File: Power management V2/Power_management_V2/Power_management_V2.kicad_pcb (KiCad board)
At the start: 4 copper layers, 76.5 x 66 mm, 60 parts, among them J2 1722861104, U1 SIC437AED, U2 SIC437AED, U3 TPS3711DDCR

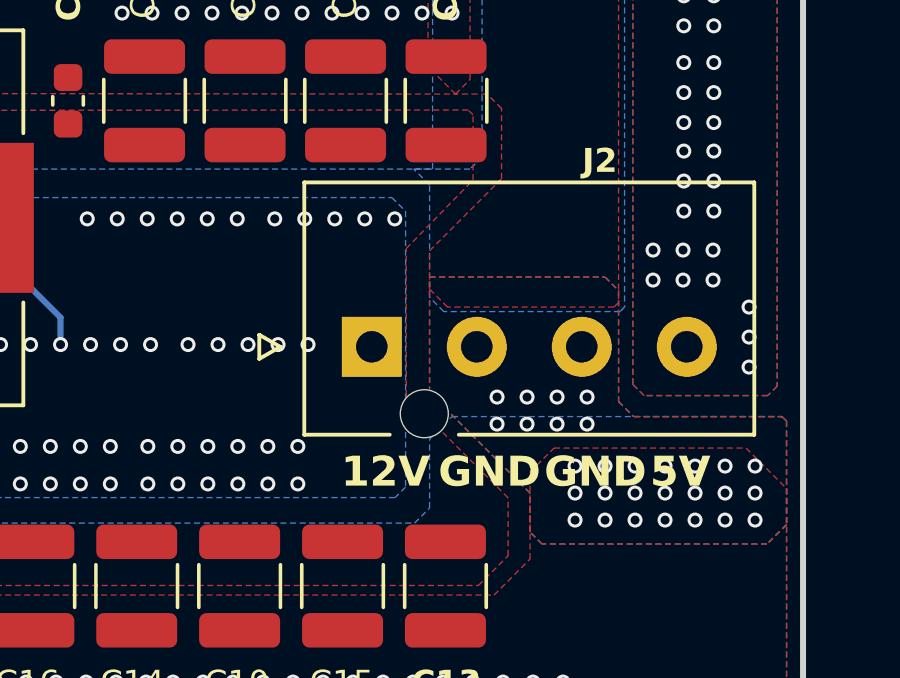
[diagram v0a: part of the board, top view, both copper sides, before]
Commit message: cap nhat 26/2
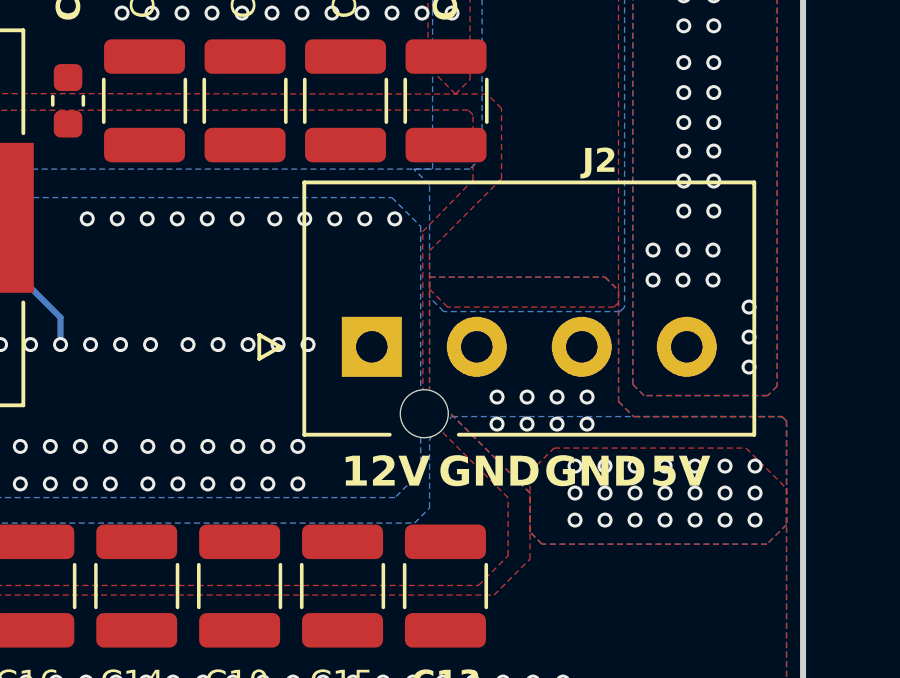
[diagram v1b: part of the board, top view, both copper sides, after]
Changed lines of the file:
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@@
 			(psa4output no)
 			(plot_black_and_white yes)
-			(plotinvisibletext no)
 			(sketchpadsonfab no)
 			(plotpadnumbers no)
@@
 			(pts
 				(xy 119.437786 84.942682) (xy 118.362 86.018468) (xy 118.362 90.8548) (xy 114.642 94.5748) (xy 114.642 99.2098)
-				(xy 116.212 100.7798) (xy 137.732 100.7798) (xy 138.722 99.7898) (xy 138.722 97.8598) (xy 135.3268 94.4646)
-				(xy 135.32325 89.551777) (xy 137.552 87.264113) (xy 137.552 85.091342) (xy 137.387926 84.93058)
+				(xy 116.212 100.7798) (xy 137.732 100.7798) (xy 138.722 99.7898) (xy 138.722 97.8598) (xy 135.880716 95.018516)
+				(xy 135.876356 88.984051) (xy 137.552 87.264113) (xy 137.552 85.091342) (xy 137.387926 84.93058)
 			)
 		)
@@
 		(polygon
 			(pts
-				(xy 120.652 87.8498) (xy 134.84575 87.8498) (xy 135.302 88.30605) (xy 135.302 97.4998) (xy 134.952 97.8498)
+				(xy 120.652 87.8498) (xy 134.84575 87.8498) (xy 135.807 88.81105) (xy 135.807 96.9948) (xy 134.952 97.8498)
 				(xy 120.407 97.8498) (xy 119.952 97.3948) (xy 119.952 88.5498)
 			)
@@
 				(xy 142.152 87.8498) (xy 142.377 88.0748) (xy 142.377 94.6498) (xy 142.877 95.1498) (xy 147.577 95.1498)
 				(xy 147.752 95.3248) (xy 147.752 107.5248) (xy 146.828349 108.448451) (xy 138.900677 108.428973)
-				(xy 135.802 105.322673) (xy 135.802 88.3748) (xy 136.327 87.8498)
+				(xy 136.092 105.613385) (xy 136.092 88.8848) (xy 137.127 87.8498)
 			)
 		)
